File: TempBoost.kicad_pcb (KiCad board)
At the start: 2 copper layers, 63 parts, among them J1 Conn_01x02, J2 Conn_01x02, Q201 Q_NMOS_GSD, SW101 SW_SPST, T101 3FD-224, U101 DF005S2, U201 MIC2920, U203 UCC27517A, U204 2925, U205 LM2904, U206 TPS1H100, U207 LM1117-5.0, U208 MAX4477

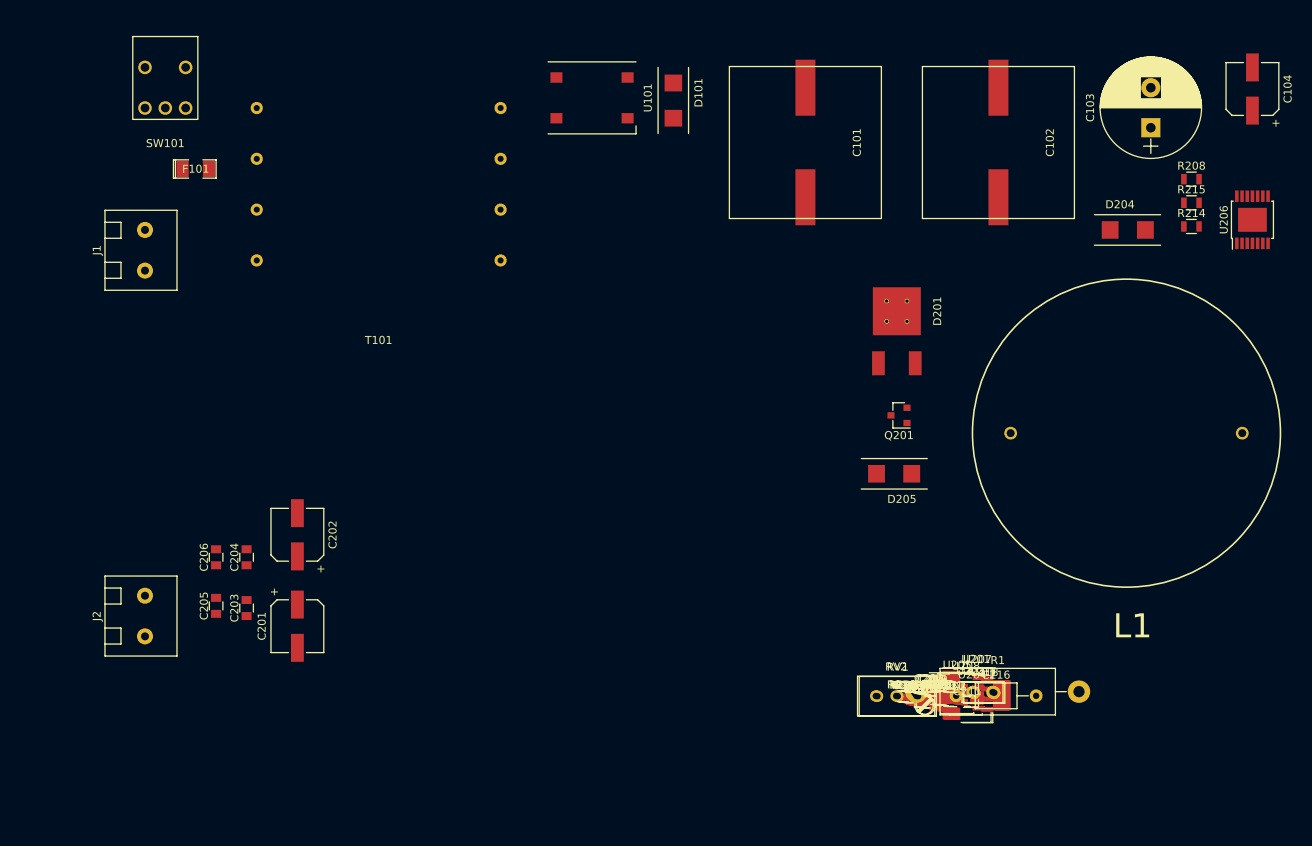
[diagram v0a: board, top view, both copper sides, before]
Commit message: Base Placement
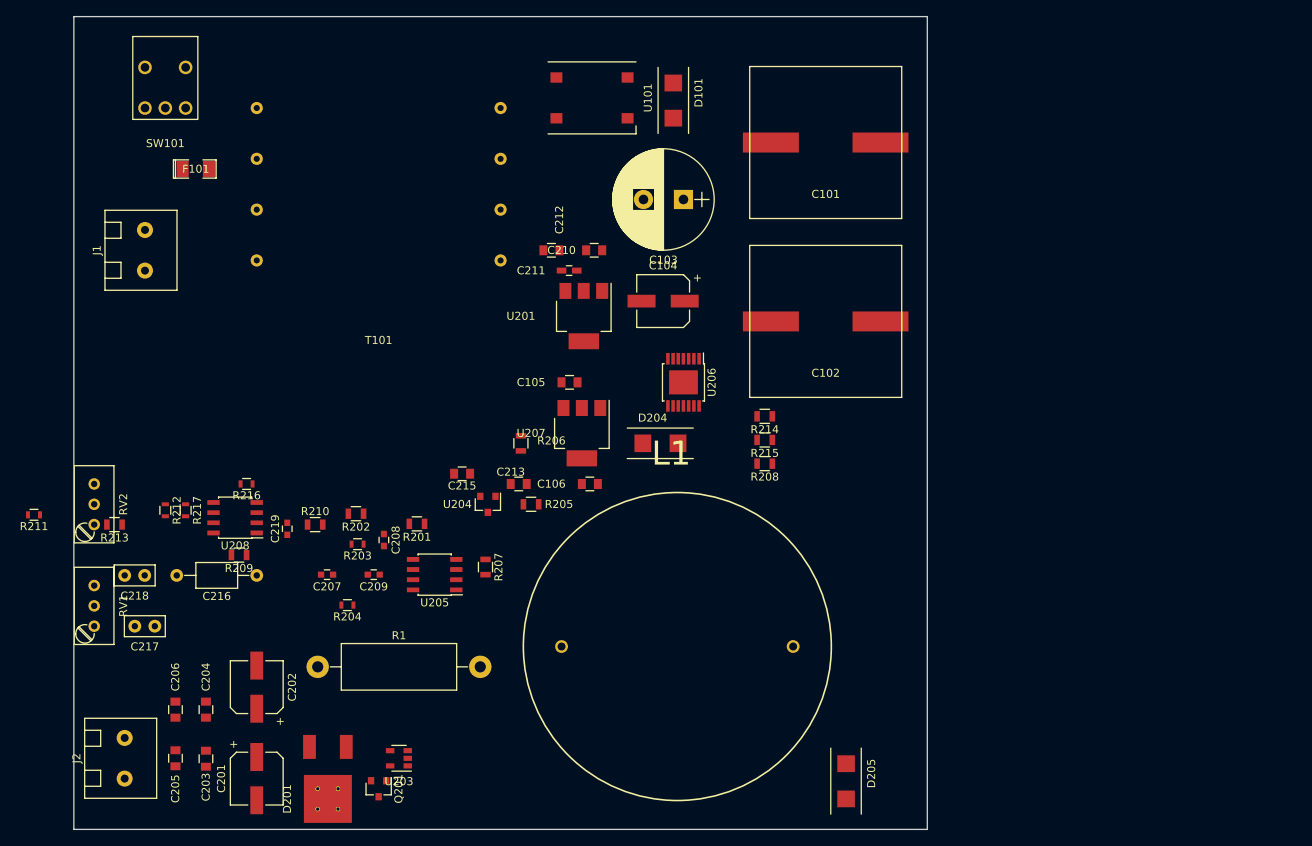
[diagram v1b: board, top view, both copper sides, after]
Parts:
- C202: value 100uF -> 100uf
- L1: value 2.2mH -> L; footprint BoostLib:1140-122K -> 1140-122K
- moved R211 111.4 mm to (38.2, 82.6), turned to 180 degrees
- moved R213 105.9 mm to (48.3, 83.8), turned to 180 degrees
- moved RV2 105.0 mm to (45.7, 83.8), turned to 270 degrees
- moved C218 104.7 mm to (52.0, 90.2), turned to 180 degrees
- moved RV1 103.4 mm to (45.7, 96.5), turned to 270 degrees
- moved C217 102.5 mm to (53.3, 96.5), turned to 180 degrees
- moved R212 95.7 mm to (54.6, 82.0), turned to 270 degrees
- moved U208 93.9 mm to (63.3, 83.0), turned to 180 degrees
- moved D201 93.7 mm to (74.9, 118.1), turned to 180 degrees
- moved R217 93.5 mm to (57.1, 82.0), turned to 270 degrees
- moved R209 89.4 mm to (63.8, 87.6), turned to 180 degrees
- moved C216 88.7 mm to (66.0, 90.2), turned to 180 degrees
- moved R216 86.0 mm to (64.8, 78.7), turned to 180 degrees
- moved C219 83.3 mm to (69.8, 84.3), turned to 90 degrees
- moved R210 81.3 mm to (73.3, 83.8)
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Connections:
- net Gate renamed GATE
- net Net-(C213-Pad1) renamed /Ref_in
- net Net-(F101-Pad2) renamed /AC_fused
- net Net-(J1-Pad1) renamed /AC_Com
- net Net-(R207-Pad2) renamed /OV_Set
- net Net-(R214-Pad2) renamed /TI_CL
- net Net-(R215-Pad2) renamed /TI_CS
- net Net-(T101-Pad5) renamed /AC+
- net Net-(T101-Pad8) renamed /AC-
- C101 pad 2: VRECT- -> GND
- C102 pad 2: VRECT- -> GND
- C103 pad 2: VRECT- -> GND
- C104 pad 2: VRECT- -> GND
- C201 pad 1: Net-(C201-Pad1) -> LOAD+
- C201 pad 2: Net-(C201-Pad2) -> GND
- C202 pad 1: Net-(C202-Pad1) -> LOAD+
- C202 pad 2: Net-(C202-Pad2) -> GND
- C203 pad 1: Net-(C203-Pad1) -> LOAD+
- C203 pad 2: Net-(C203-Pad2) -> GND
- C204 pad 1: Net-(C204-Pad1) -> LOAD+
- C204 pad 2: Net-(C204-Pad2) -> GND
- C205 pad 1: Net-(C205-Pad1) -> LOAD+
- C205 pad 2: Net-(C205-Pad2) -> GND
- C206 pad 1: Net-(C206-Pad1) -> LOAD+
- C206 pad 2: Net-(C206-Pad2) -> GND
- C210 pad 2: VRECT- -> Net-(C210-Pad2)
- C211 pad 2: VRECT- -> Net-(C210-Pad2)
- C212 pad 2: VRECT- -> Net-(C210-Pad2)
- D101 pad 2: VRECT- -> GND
- D201 pad 1: Net-(D201-Pad1) -> LOAD+
- D201 pad 2: Net-(D201-Pad2) -> /I_Side
- D204 pad 1: Net-(D204-Pad1) -> VSWITCHED
- D204 pad 2: Net-(D204-Pad2) -> /I_Side
- D205 pad 1: Net-(D205-Pad1) -> VSWITCHED
- D205 pad 2: Net-(D205-Pad2) -> GND
- Q201 pad 3: Net-(Q201-Pad3) -> /I_Side
- U101 pad 2: VRECT- -> GND
- U203 pad 2: VRECT- -> GND
- U203 pad 4: VRECT- -> GND
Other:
- board outline added: 106.7 x 101.6 mm
- board text added: "R1 = optional gate resistor? Change to 33 Ohm 0805 if I can change the BOM"
